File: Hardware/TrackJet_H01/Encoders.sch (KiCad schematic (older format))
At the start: 30 parts, among them U10 TCRT5000, U11 TCRT5000, U12 TCRT5000, U7 TCRT5000, U8 TCRT5000, U9 TCRT5000

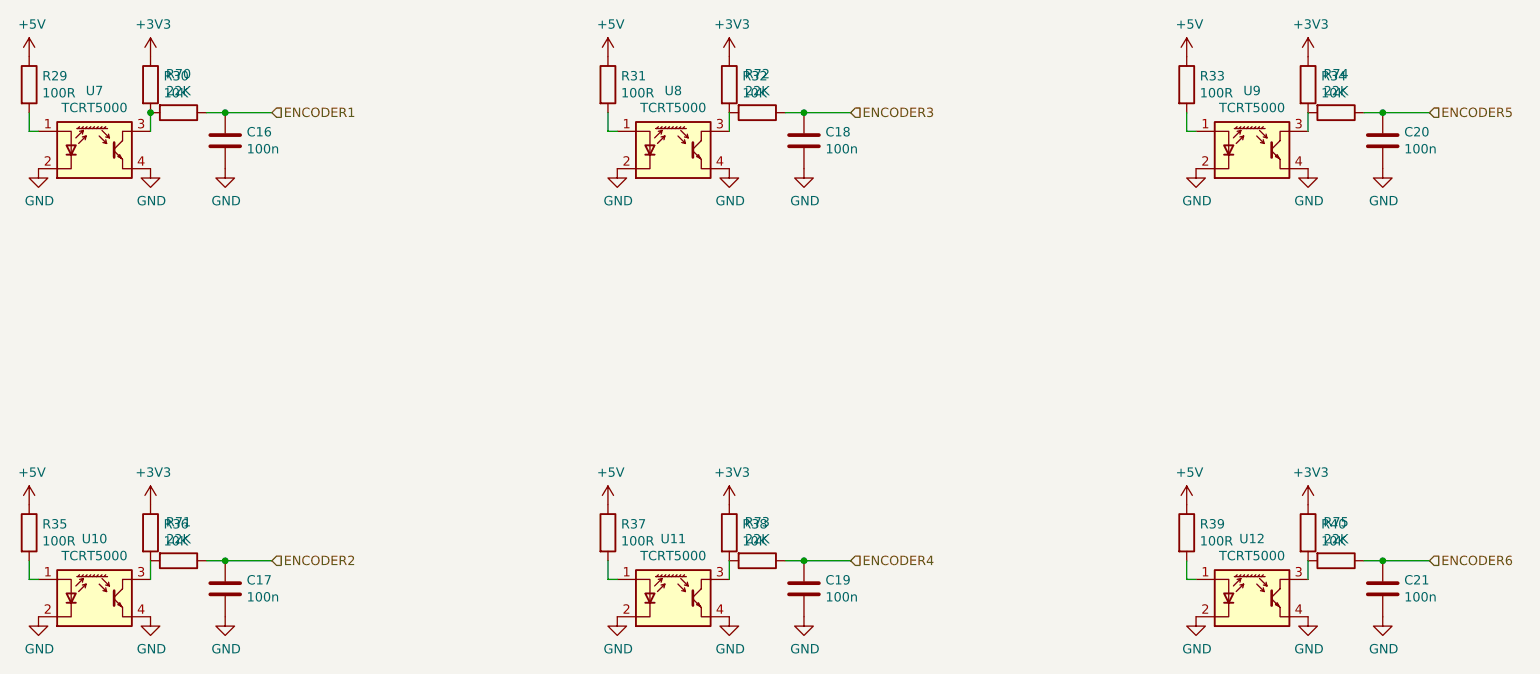
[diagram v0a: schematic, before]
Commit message: Updated H01 PCB
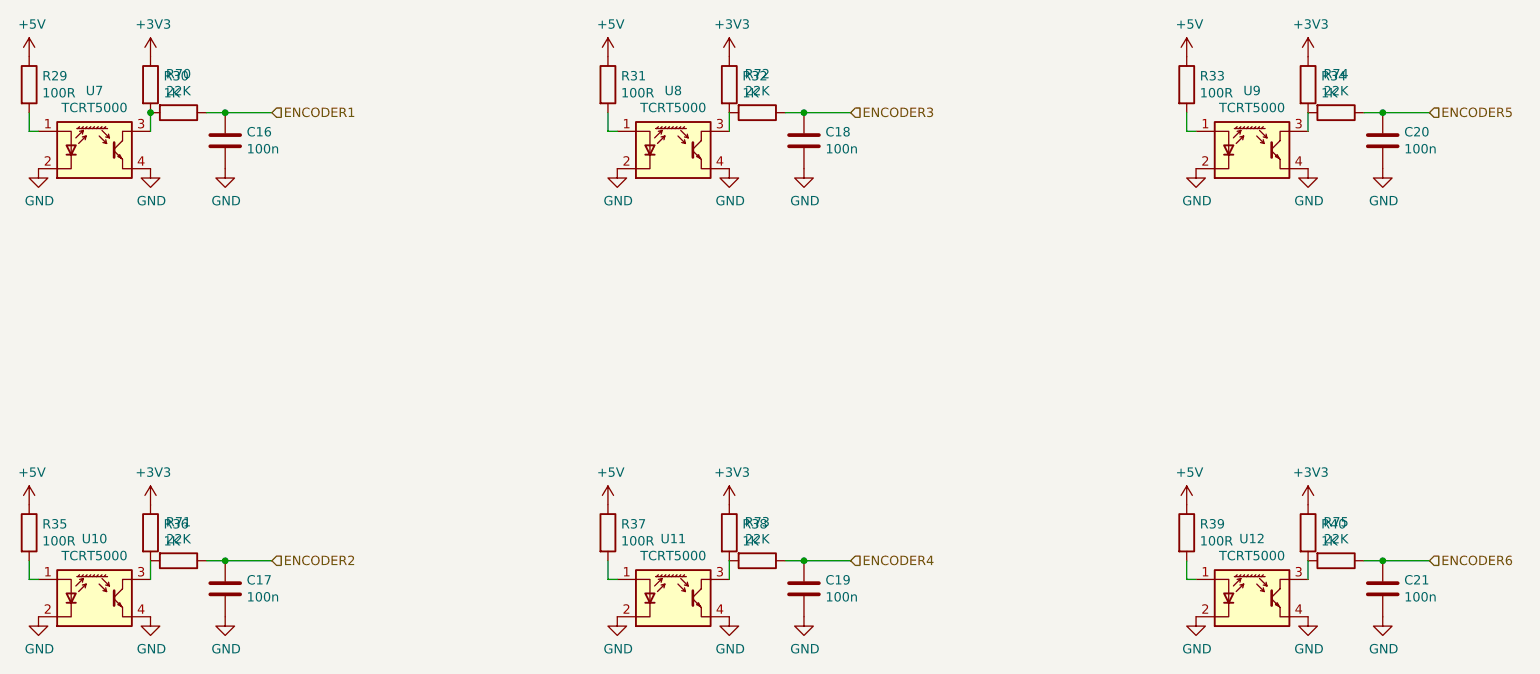
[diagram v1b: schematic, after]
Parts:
- R30, R32, R34, R36, R38, R40: value 10K -> 1K; LCSC C25804 -> C21190
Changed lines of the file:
@@
 P 3250 3100
 F 0 "R30" H 3320 3146 50  0000 L CNN
-F 1 "10K" H 3320 3055 50  0000 L CNN
+F 1 "1K" H 3320 3055 50  0000 L CNN
 F 2 "Resistor_SMD:R_0603_1608Metric" V 3180 3100 50  0001 C CNN
 F 3 "~" H 3250 3100 50  0001 C CNN
-F 4 "C25804" H 3250 3100 50  0001 C CNN "LCSC"
+F 4 "C21190" H 3250 3100 50  0001 C CNN "LCSC"
 	1    3250 3100
 	1    0    0    -1
@@
 P 3250 5500
 F 0 "R36" H 3320 5546 50  0000 L CNN
-F 1 "10K" H 3320 5455 50  0000 L CNN
+F 1 "1K" H 3320 5455 50  0000 L CNN
 F 2 "Resistor_SMD:R_0603_1608Metric" V 3180 5500 50  0001 C CNN
 F 3 "~" H 3250 5500 50  0001 C CNN
-F 4 "C25804" H 3250 5500 50  0001 C CNN "LCSC"
+F 4 "C21190" H 3250 5500 50  0001 C CNN "LCSC"
 	1    3250 5500
 	1    0    0    -1
@@
 P 6350 3100
 F 0 "R32" H 6420 3146 50  0000 L CNN
-F 1 "10K" H 6420 3055 50  0000 L CNN
+F 1 "1K" H 6420 3055 50  0000 L CNN
 F 2 "Resistor_SMD:R_0603_1608Metric" V 6280 3100 50  0001 C CNN
 F 3 "~" H 6350 3100 50  0001 C CNN
-F 4 "C25804" H 6350 3100 50  0001 C CNN "LCSC"
+F 4 "C21190" H 6350 3100 50  0001 C CNN "LCSC"
 	1    6350 3100
 	1    0    0    -1
@@
 P 6350 5500
 F 0 "R38" H 6420 5546 50  0000 L CNN
-F 1 "10K" H 6420 5455 50  0000 L CNN
+F 1 "1K" H 6420 5455 50  0000 L CNN
 F 2 "Resistor_SMD:R_0603_1608Metric" V 6280 5500 50  0001 C CNN
 F 3 "~" H 6350 5500 50  0001 C CNN
-F 4 "C25804" H 6350 5500 50  0001 C CNN "LCSC"
+F 4 "C21190" H 6350 5500 50  0001 C CNN "LCSC"
 	1    6350 5500
 	1    0    0    -1
@@
 P 9450 3100
 F 0 "R34" H 9520 3146 50  0000 L CNN
-F 1 "10K" H 9520 3055 50  0000 L CNN
+F 1 "1K" H 9520 3055 50  0000 L CNN
 F 2 "Resistor_SMD:R_0603_1608Metric" V 9380 3100 50  0001 C CNN
 F 3 "~" H 9450 3100 50  0001 C CNN
-F 4 "C25804" H 9450 3100 50  0001 C CNN "LCSC"
+F 4 "C21190" H 9450 3100 50  0001 C CNN "LCSC"
 	1    9450 3100
 	1    0    0    -1
@@
 P 9450 5500
 F 0 "R40" H 9520 5546 50  0000 L CNN
-F 1 "10K" H 9520 5455 50  0000 L CNN
+F 1 "1K" H 9520 5455 50  0000 L CNN
 F 2 "Resistor_SMD:R_0603_1608Metric" V 9380 5500 50  0001 C CNN
 F 3 "~" H 9450 5500 50  0001 C CNN
-F 4 "C25804" H 9450 5500 50  0001 C CNN "LCSC"
+F 4 "C21190" H 9450 5500 50  0001 C CNN "LCSC"
 	1    9450 5500
 	1    0    0    -1
